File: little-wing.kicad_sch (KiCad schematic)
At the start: 132 parts, among them IC1 AP7335-WG-7, J1 nice!view, J10 rgb, J11 rows, J12 columns, J13 columns, J2 Battery, J3 trackball, J4 rotary, J5 trackball, J6 nice!view, J7 Battery, J8 rgb, J9 rows, SW1 Power, SW2 Reset, SW3 Reset, SW4 Power, U1 nice!nano v2, U2 PMW3610, U3 nice!nano v2

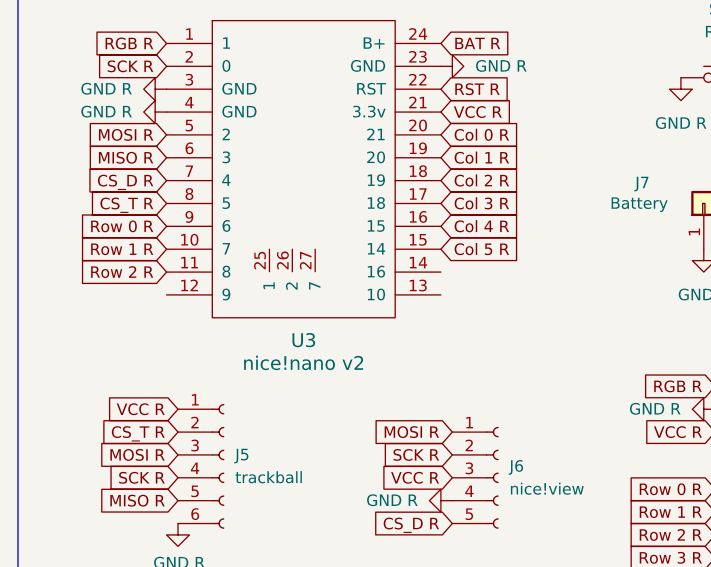
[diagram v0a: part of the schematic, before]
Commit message: Wiring together the mobos
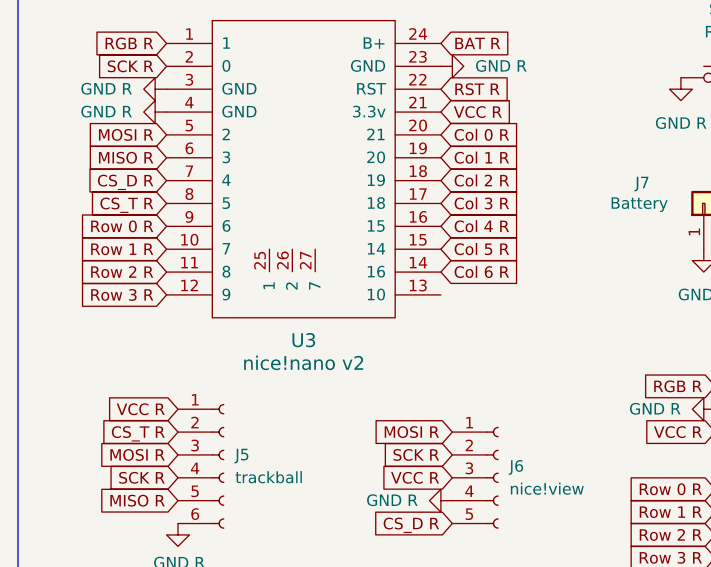
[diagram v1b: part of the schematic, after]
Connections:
- net CS_T  L is gone; now on net CS_T L: J4.2 (Pin_2)
- net SCK  L is gone; now on net SCK L: J4.4 (Pin_4)
- net Col 6 R: now also U3.14 (16)
- net Row 3 R: now also U3.12 (9)
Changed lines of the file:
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@@
 		)
 	)
-	(global_label "CS_T  L"
+	(global_label "CS_T L"
 		(shape input)
 		(at 36.83 67.31 180)
@@
 		)
 		(property "Intersheetrefs" "${INTERSHEET_REFS}"
-			(at 26.4668 67.31 0)
+			(at 27.4344 67.31 0)
 			(effects
 				(font
@@
 		)
 	)
-	(global_label "SCK  L"
+	(global_label "SCK L"
 		(shape input)
 		(at 36.83 72.39 180)
@@
 		)
 		(property "Intersheetrefs" "${INTERSHEET_REFS}"
-			(at 27.132 72.39 0)
+			(at 28.0996 72.39 0)
 			(effects
 				(font
@@
 		)
 	)
+	(global_label "Col 6 R"
+		(shape input)
+		(at 66.04 134.62 0)
+		(fields_autoplaced yes)
+		(effects
+			(font
+				(size 1.27 1.27)
+			)
+			(justify left)
+		)
+		(property "Intersheetrefs" "${INTERSHEET_REFS}"
+			(at 76.5241 134.62 0)
+			(effects
+				(font
+					(size 1.27 1.27)
+				)
+				(justify left)
+				(hide yes)
+			)
+		)
+	)
 	(global_label "Row 2 R"
 		(shape input)
@@
 			(effects
 				(font
+					(size 1.27 1.27)
+				)
+				(justify right)
+				(hide yes)
+			)
+		)
+	)
+	(global_label "Row 3 R"
+		(shape input)
+		(at 35.56 137.16 180)
+		(fields_autoplaced yes)
+		(effects
+			(font
+				(size 1.27 1.27)
+			)
+			(justify right)
+		)
+		(property "Intersheetrefs" "${INTERSHEET_REFS}"
+			(at 24.4106 137.16 0)
+			(effects
+				(font
